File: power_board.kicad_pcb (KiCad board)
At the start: 2 copper layers, 87.2 x 64 mm, 66 parts, among them J1 Conn_01x01, J10 Conn_01x01, J11 Conn_01x01, J12 Conn_01x01, J13 Conn_01x01, J14 Conn_01x01, J15 Conn_01x01, J16 Conn_01x01, J17 Conn_01x03, J18 Conn_01x03, J19 Conn_01x03, J2 Conn_01x01, J20 Conn_01x02, J21 Conn_01x02, J22 Conn_01x02, J3 Conn_01x01, J4 Conn_01x01, J5 Conn_01x01, J6 Conn_01x01, J7 Conn_01x01, J8 Conn_01x01, J9 Conn_01x01, Q1 IRF540S, Q2 IRF540S, Q3 IRF540S, Q4 IRF540S, U1 TPS54561, U2 TPS54561

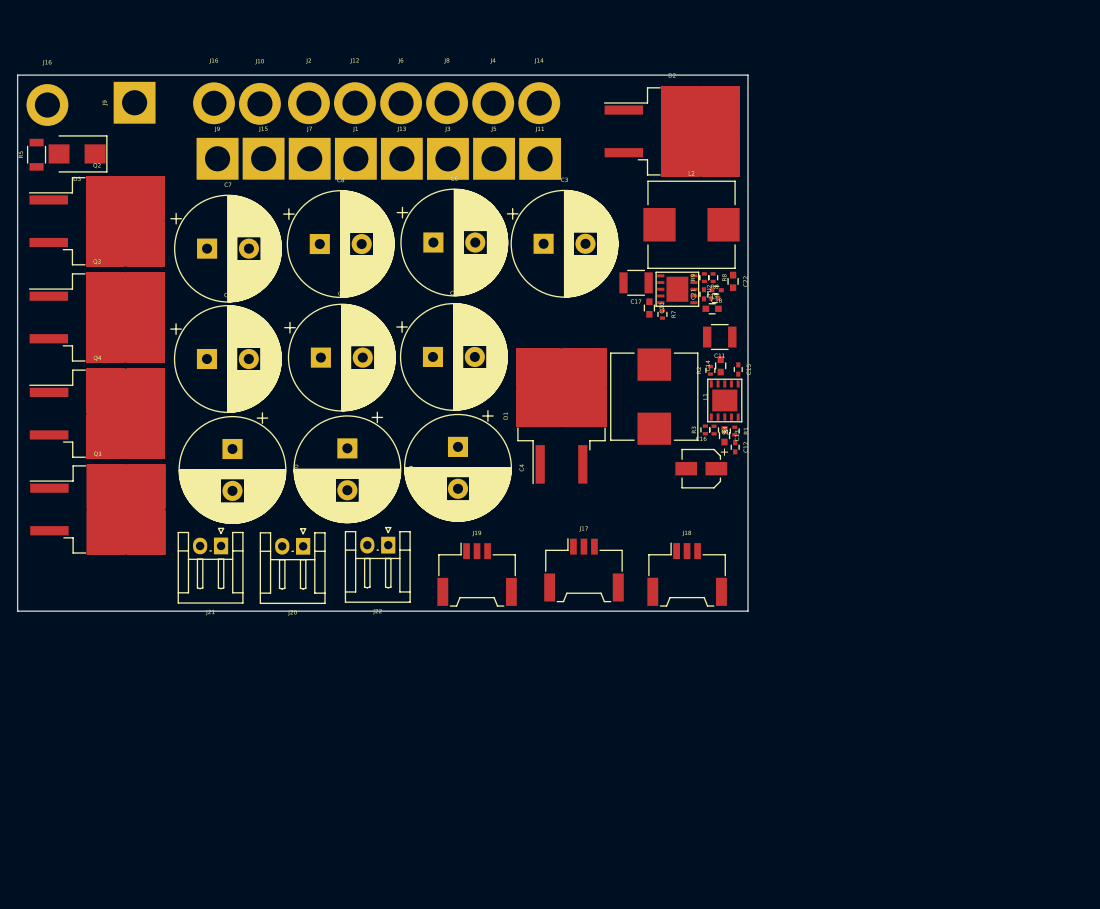
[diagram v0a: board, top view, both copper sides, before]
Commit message: new pcb design
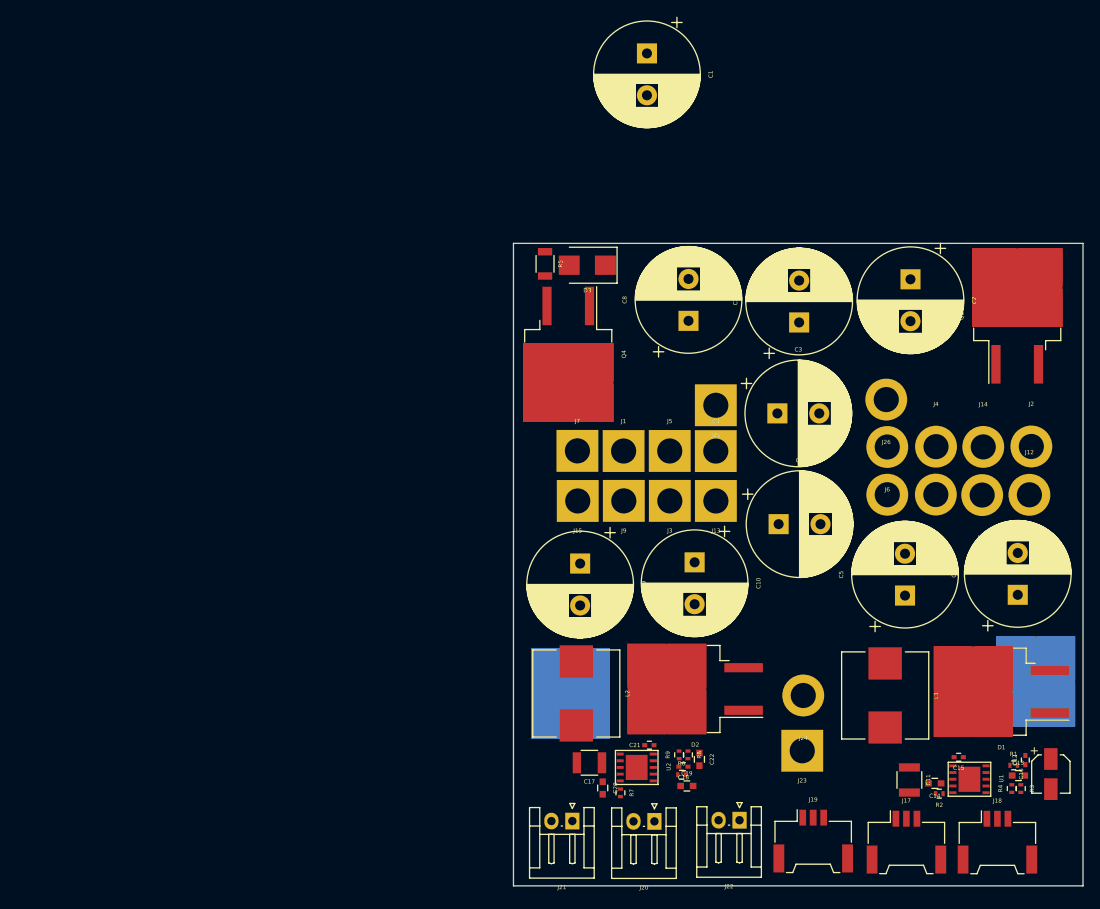
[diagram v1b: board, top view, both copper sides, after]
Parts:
- removed the J16 at (54.4, 26.6)
- removed the J9 at (65.3, 26.3)
- added J23: Conn_01x01, MB_LIB:via_sq, F.Cu at (144.5, 103.2)
- added J24: Conn_01x01, MB_LIB:via, F.Cu at (144.6, 97.1)
- added J25: Conn_01x01, MB_LIB:via_sq, F.Cu at (134.2, 61.9)
- added J26: Conn_01x01, MB_LIB:via, F.Cu at (154.5, 61.7)
- Q2, Q3: moved to B.Cu
- moved Q2 121.8 mm to (169.0, 95.4)
- moved Q1 112.2 mm to (170.1, 51.8), turned to 90 degrees
- moved J10 98.1 mm to (166.0, 73.1), turned to 0 degrees
- moved J2 95.5 mm to (171.8, 67.3)
- moved J12 93.1 mm to (171.6, 73.1)
- moved J16 93.0 mm to (154.6, 73.1), turned to 0 degrees
- moved C2 84.5 mm to (157.4, 47.4), turned to 270 degrees
- moved Q3 74.9 mm to (120.2, 96.8), turned to 180 degrees
- moved J8 74.8 mm to (160.4, 73.1), turned to 0 degrees
- moved C7 71.2 mm to (144.1, 52.5), turned to 90 degrees
- moved J6 71.1 mm to (154.6, 67.4), turned to 0 degrees
- moved C4 69.1 mm to (170.2, 85.0), turned to 90 degrees
- moved J14 67.0 mm to (166.1, 67.4)
- moved J4 66.9 mm to (160.4, 67.4)
- moved D2 66.6 mm to (131.7, 96.3), turned to 180 degrees
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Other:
- board size 87.2 x 64 mm -> 68 x 76.7 mm
